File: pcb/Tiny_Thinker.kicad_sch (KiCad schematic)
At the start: 43 parts, among them J1 Conn_02x20_Odd_Even, J2 Conn_02x20_Odd_Even, J3 SWD, J4 SPI1, J5 I2C1_A, J6 I2C1_B, J8 USB_C_Receptacle_USB2.0_16P, SW1 SW_Push, SW2 SW_SPDT, U1 STM32F446RET6, U2 AMS1117-3.3, U3 USBLC6-2SC6, Y1 16MHz

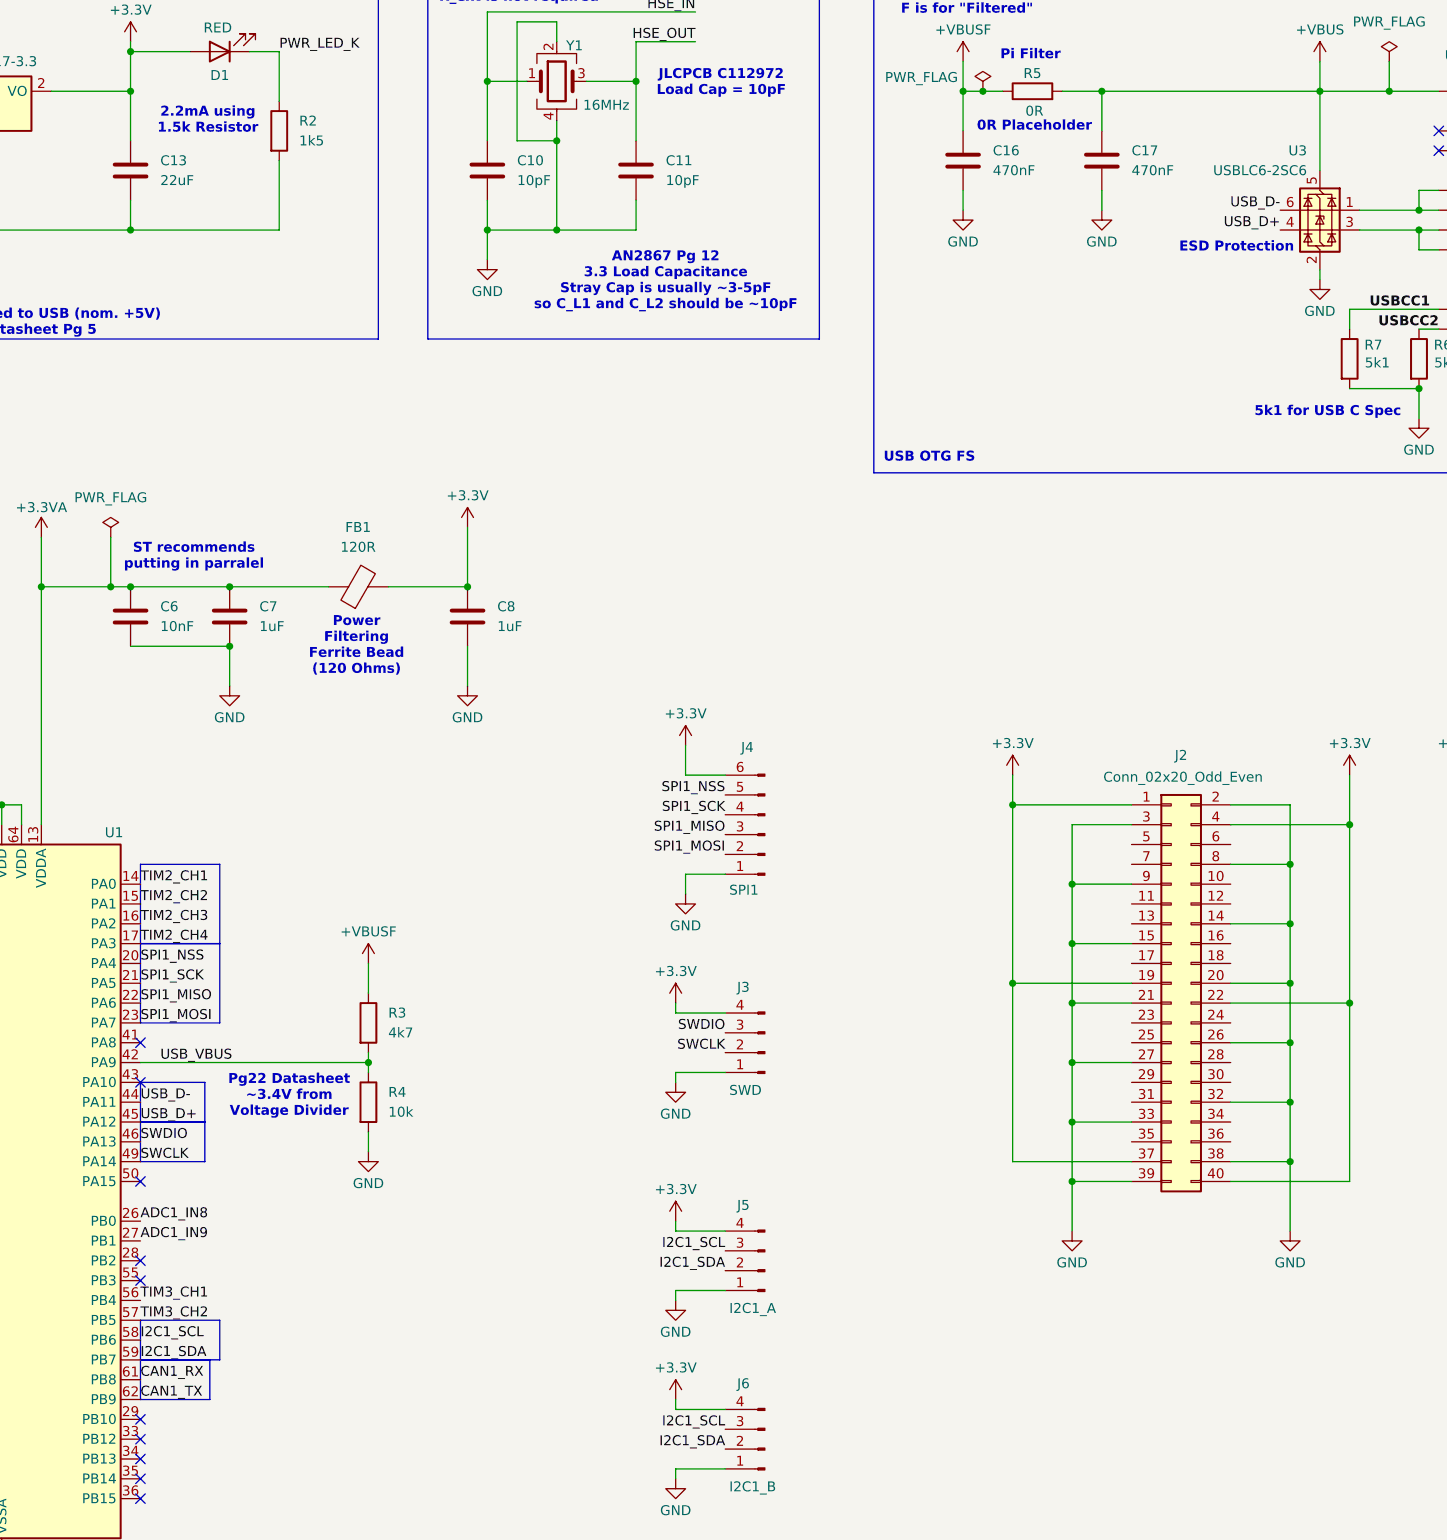
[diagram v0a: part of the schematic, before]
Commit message: gave colors to all netclasses
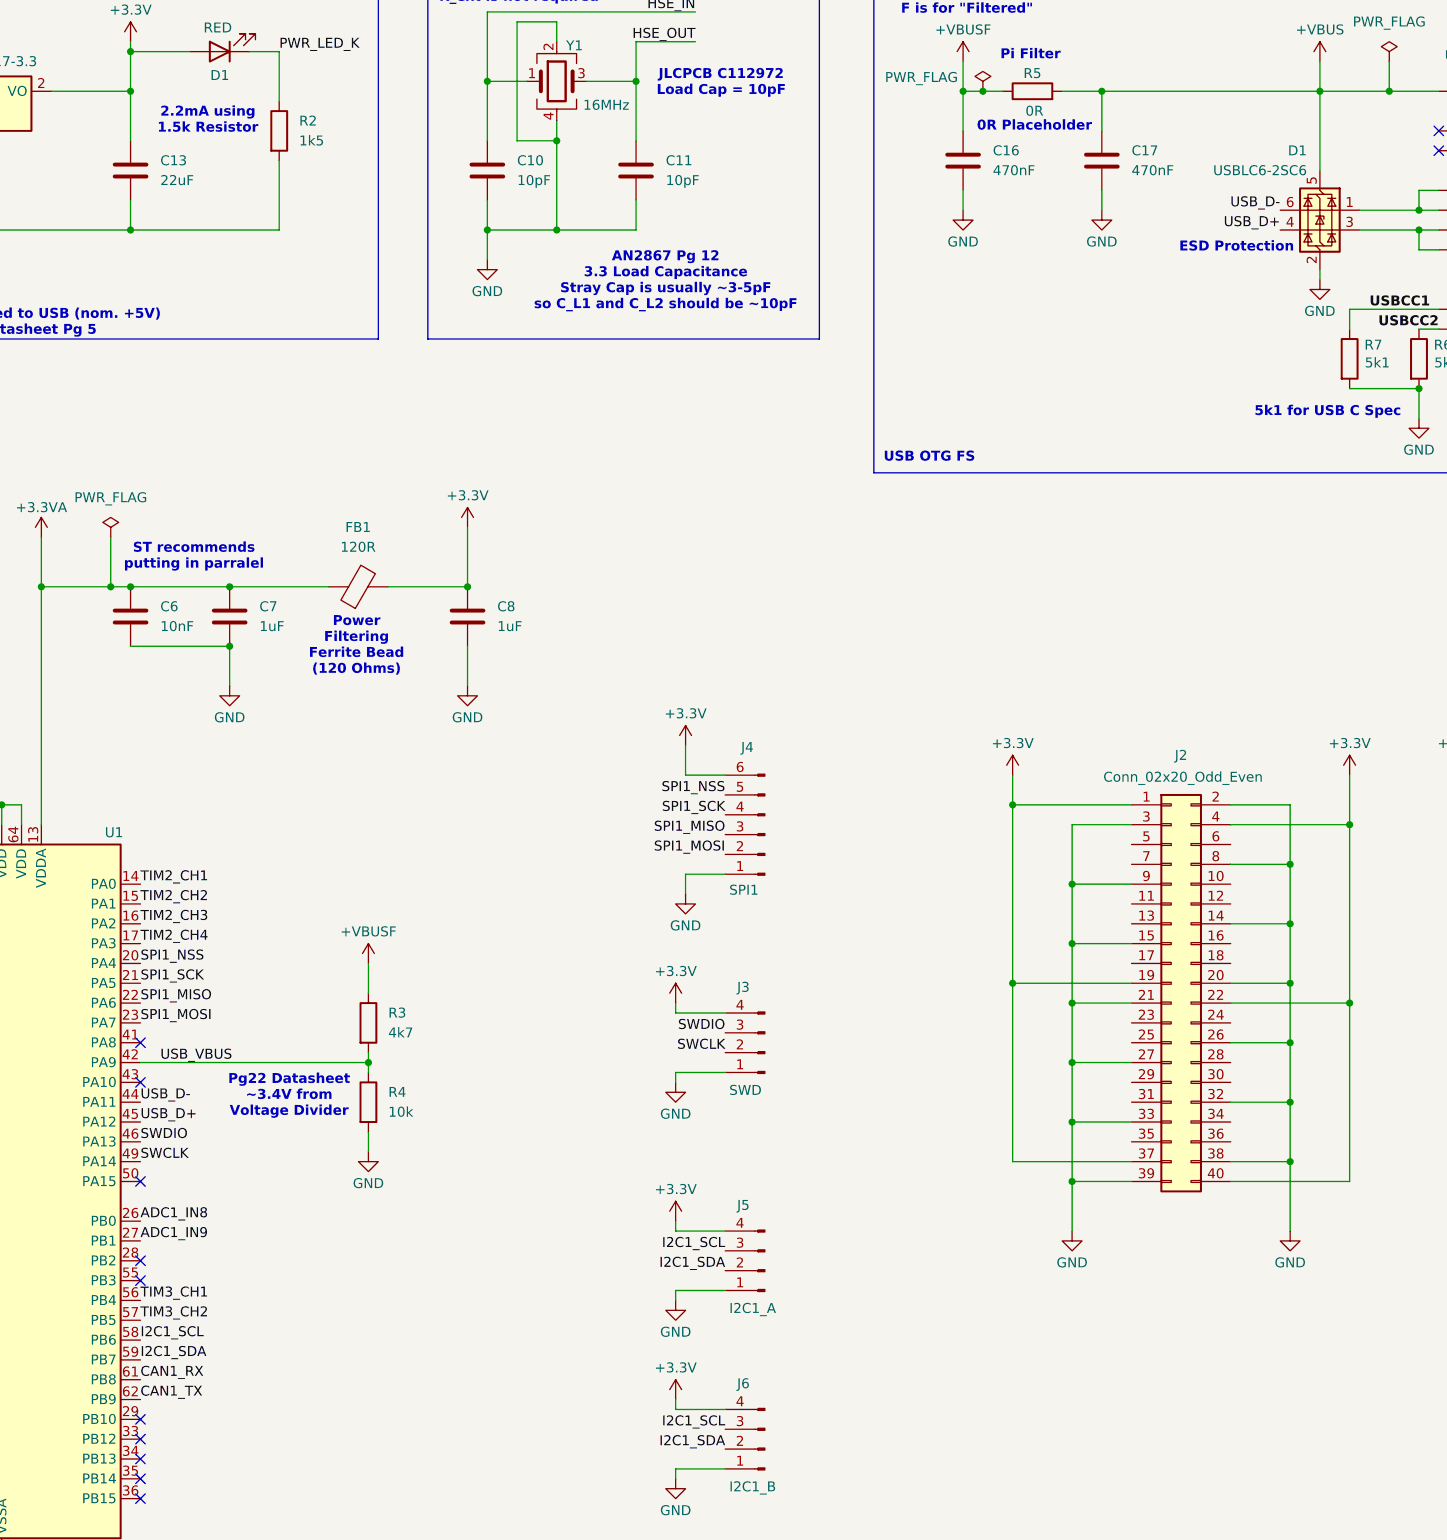
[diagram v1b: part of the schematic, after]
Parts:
- renumbered U3 to D1
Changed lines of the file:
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@@
 	)
 	(rectangle
-		(start 168.91 199.39)
-		(end 179.07 204.47)
-		(stroke
-			(width 0)
-			(type default)
-		)
-		(fill
-			(type none)
-		)
-	)
-	(rectangle
 		(start 205.74 21.59)
 		(end 255.905 73.66)
@@
 	)
 	(rectangle
-		(start 168.91 173.99)
-		(end 177.165 179.07)
-		(stroke
-			(width 0)
-			(type default)
-		)
-		(fill
-			(type none)
-		)
-	)
-	(rectangle
-		(start 168.91 140.97)
-		(end 179.07 151.13)
-		(stroke
-			(width 0)
-			(type default)
-		)
-		(fill
-			(type none)
-		)
-	)
-	(rectangle
-		(start 168.91 151.13)
-		(end 179.07 161.29)
-		(stroke
-			(width 0)
-			(type default)
-		)
-		(fill
-			(type none)
-		)
-	)
-	(rectangle
-		(start 168.91 168.91)
-		(end 177.165 173.99)
-		(stroke
-			(width 0)
-			(type default)
-		)
-		(fill
-			(type none)
-		)
-	)
-	(rectangle
 		(start 262.89 21.59)
 		(end 367.538 90.805)
@@
 		)
 	)
-	(rectangle
-		(start 168.91 204.47)
-		(end 177.8 209.55)
-		(stroke
-			(width 0)
-			(type default)
-		)
-		(fill
-			(type none)
-		)
-	)
 	(text "Tiny Thinker STM32 PCB\n"
 		(exclude_from_sim no)
@@
 		(on_board yes)
 		(dnp no)
-		(property "Reference" "U3"
+		(property "Reference" "D1"
 			(at 318.3889 49.53 0)
 			(effects
@@
 			(project ""
 				(path "/1492d82e-cea7-4984-859f-7eb0a1e67ad8"
-					(reference "U3")
+					(reference "D1")
 					(unit 1)
 				)
